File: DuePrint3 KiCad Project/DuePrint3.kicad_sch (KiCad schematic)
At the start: 49 parts, among them J1 MF3.0-2x12-430452412, J10 436500215, J11 M20-9990245, J12 M20-9990245, J13 EHT-125-01-S-D, J14 EHT-110-01-S-D, J15 EHT-125-01-S-D, J2 PPPC161LFBN-RC, J3 PPPC161LFBN-RC, J4 6P2C, J5 6P2C, J6 M20-9990345, J7 436500215, J8 436500815, J9 MF3.0-2x9-430451812, U1 SN74AHCT125DR

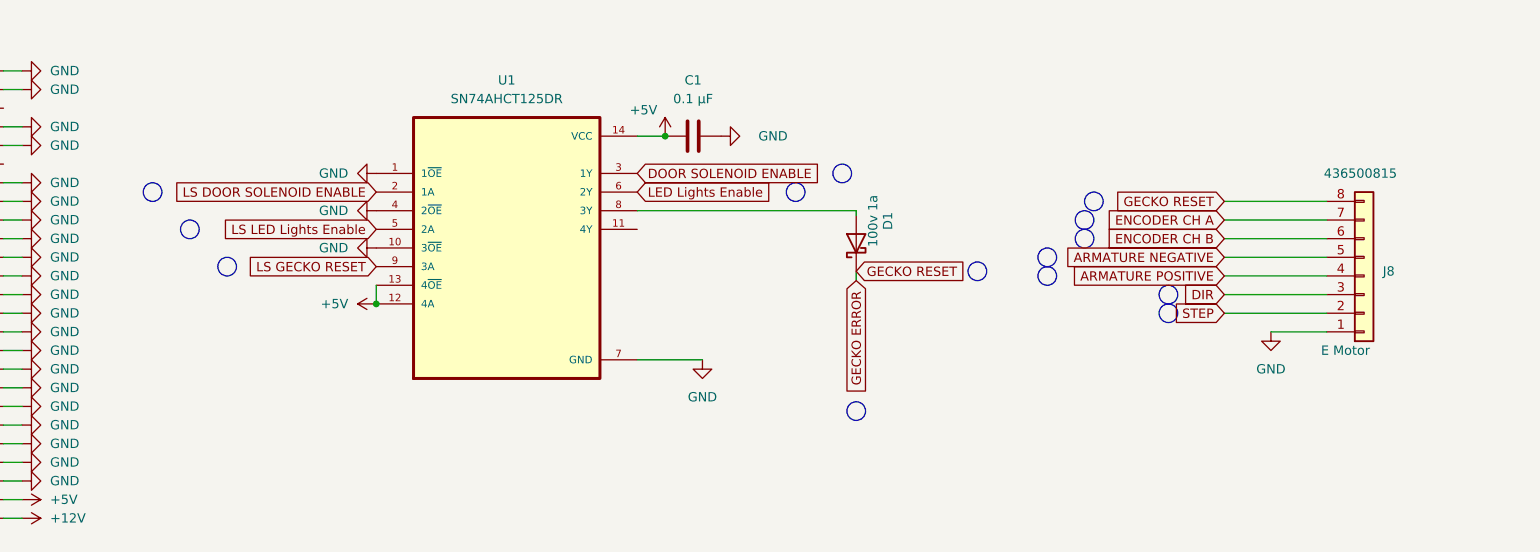
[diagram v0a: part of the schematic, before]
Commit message: Level shifter
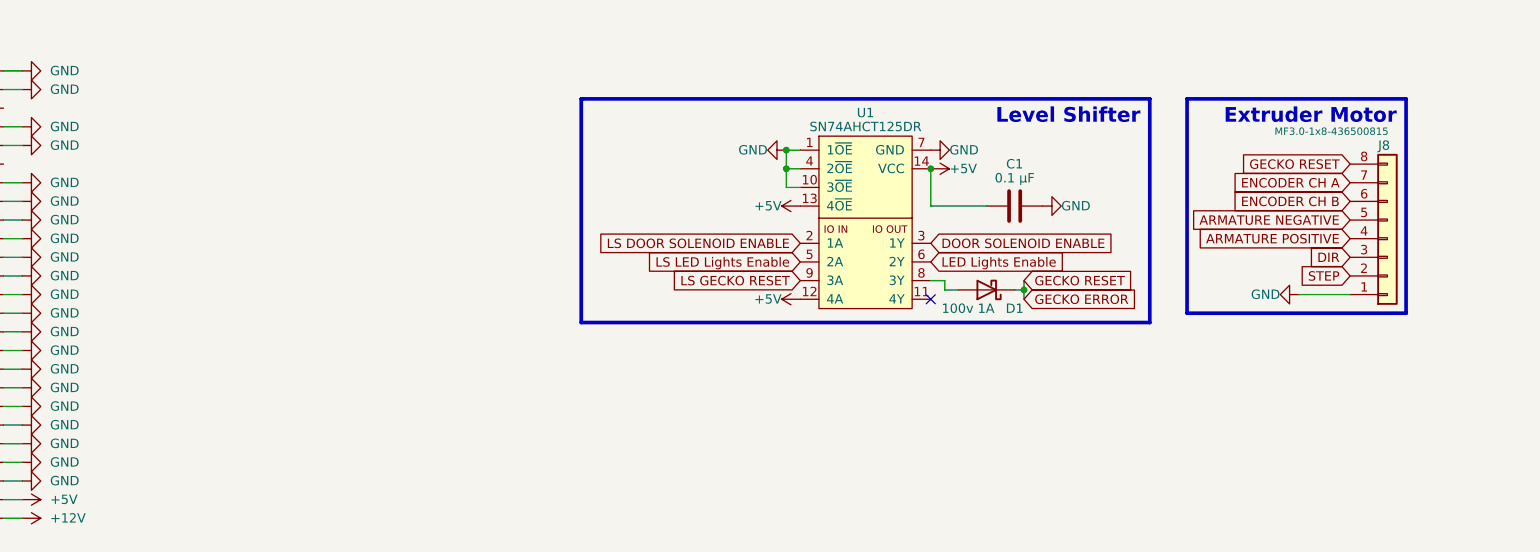
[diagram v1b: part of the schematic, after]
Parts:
- D1: value 100v 1a -> 100v 1A
- J8: value 436500815 -> MF3.0-1x8-436500815; Device E Motor -> (none)
- U1: footprint Stratasys Adapter:SOIC127P600X175-14N -> PCM_Package_SO_AKL:SOIC-14_3.9x8.7mm_P1.27mm
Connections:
- no-connect marks 10 -> 11
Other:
- note added: "Extruder Motor"
- note added: "Level Shifter"
- moved on the sheet: C1, D1, J8

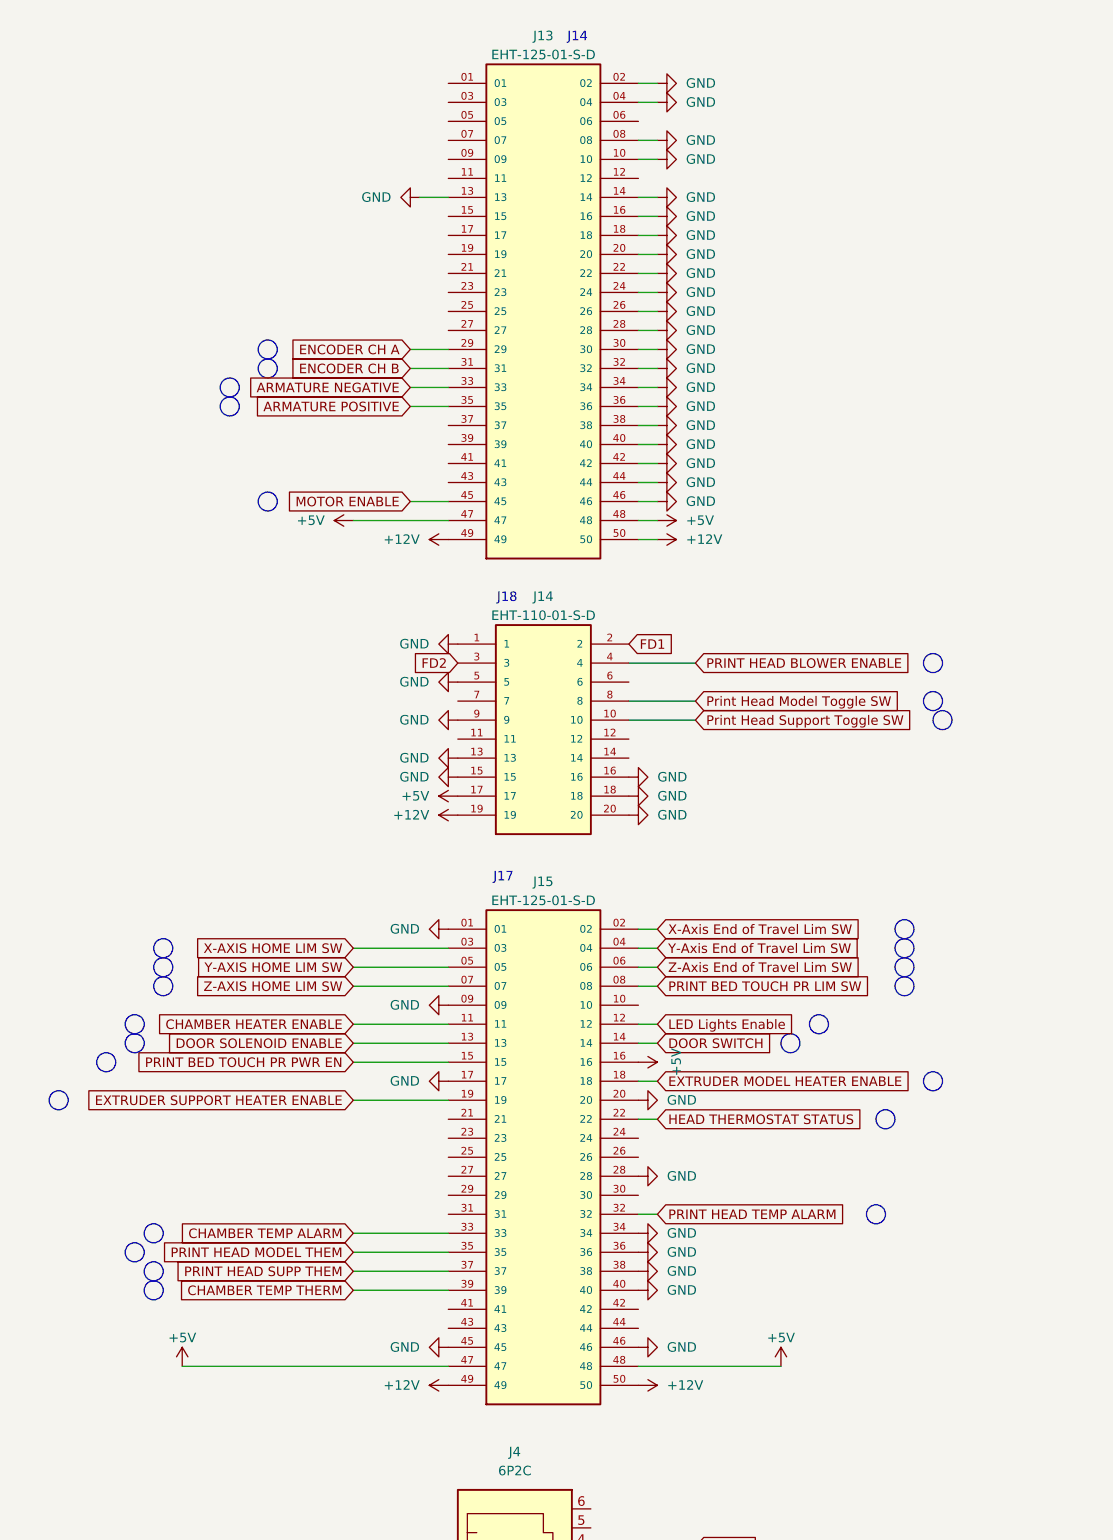
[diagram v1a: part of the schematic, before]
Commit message: PDB Connectors
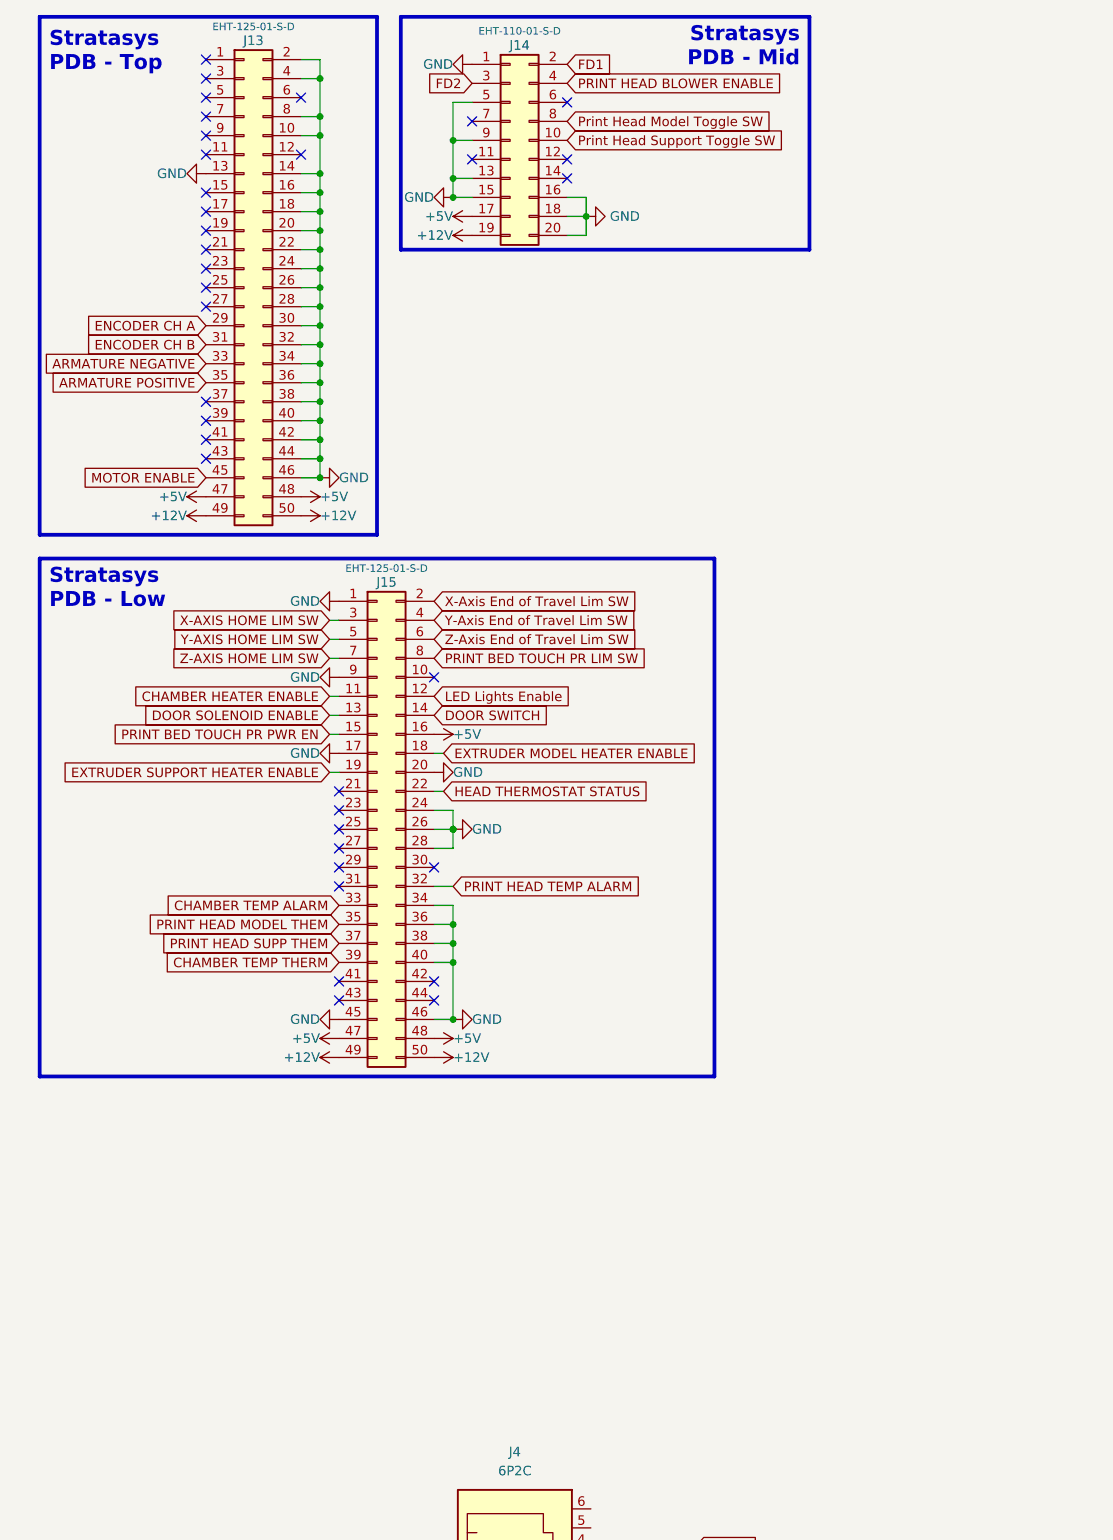
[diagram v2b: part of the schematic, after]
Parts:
- removed J13, J15: EHT-125-01-S-D, EHT-125-01-S-D:SAMTEC_EHT-125-01-S-D, symbol EHT-125-01-S-D:EHT-125-01-S-D
- removed J14: EHT-110-01-S-D, EHT-110-01-XX-D:EHT-110-01-XX-D, symbol EHT-110-01-XX-D:EHT-110-01-XX-D
- added J13, J15: EHT-125-01-S-D, EHT-125-01-S-D:SAMTEC_EHT-125-01-S-D, symbol Connector_Generic:Conn_02x25_Odd_Even
- added J14: EHT-110-01-S-D, EHT-110-01-XX-D:EHT-110-01-XX-D, symbol Connector_Generic:Conn_02x10_Odd_Even
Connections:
- net +12V: now also J13.49 (Pin_49), J13.50 (Pin_50), J14.19 (Pin_19), J15.49 (Pin_49), J15.50 (Pin_50)
- net +5V: now also J13.47 (Pin_47), J13.48 (Pin_48), J14.17 (Pin_17), J15.16 (Pin_16), J15.47 (Pin_47), J15.48 (Pin_48)
- net ARMATURE NEGATIVE: now also J13.33 (Pin_33)
- net ARMATURE POSITIVE: now also J13.35 (Pin_35)
- net CHAMBER HEATER ENABLE: now also J15.11 (Pin_11)
- net CHAMBER TEMP ALARM: now also J15.33 (Pin_33)
- net CHAMBER TEMP THERM: now also J15.39 (Pin_39)
- net DOOR SOLENOID ENABLE: now also J15.13 (Pin_13)
- net DOOR SWITCH: now also J15.14 (Pin_14)
- net EMHE PWM: now also J15.18 (Pin_18)
- net ENCODER CH A: now also J13.29 (Pin_29)
- net ENCODER CH B: now also J13.31 (Pin_31)
- net ESHE PWM: now also J15.19 (Pin_19)
- net FD1: now also J14.2 (Pin_2)
- net FD2: now also J14.3 (Pin_3)
- net GND: now also J13.10 (Pin_10), J13.13 (Pin_13), J13.14 (Pin_14), J13.16 (Pin_16), J13.18 (Pin_18), J13.2 (Pin_2), J13.20 (Pin_20), J13.22 (Pin_22), J13.24 (Pin_24), J13.26 (Pin_26), J13.28 (Pin_28), J13.30 (Pin_30), J13.32 (Pin_32), J13.34 (Pin_34), J13.36 (Pin_36), J13.38 (Pin_38), J13.4 (Pin_4), J13.40 (Pin_40), J13.42 (Pin_42), J13.44 (Pin_44), J13.46 (Pin_46), J13.8 (Pin_8), J14.1 (Pin_1), J14.13 (Pin_13), J14.15 (Pin_15), J14.16 (Pin_16), J14.18 (Pin_18), J14.20 (Pin_20), J14.5 (Pin_5), J14.9 (Pin_9), J15.1 (Pin_1), J15.17 (Pin_17), J15.20 (Pin_20), J15.24 (Pin_24), J15.26 (Pin_26), J15.28 (Pin_28), J15.34 (Pin_34), J15.36 (Pin_36), J15.38 (Pin_38), J15.40 (Pin_40), J15.45 (Pin_45), J15.46 (Pin_46), J15.9 (Pin_9)
- net HEAD THERMOSTAT STATUS: now also J15.22 (Pin_22)
- net LED Lights Enable: now also J15.12 (Pin_12)
- net MOTOR ENABLE: now also J13.45 (Pin_45)
- net PBTPE PWM: now also J15.15 (Pin_15)
- net PHBE PWM: now also J14.4 (Pin_4)
- net PRINT BED TOUCH PR LIM SW: now also J15.8 (Pin_8)
- net PRINT HEAD MODEL THEM: now also J15.35 (Pin_35)
- net PRINT HEAD SUPP THEM: now also J15.37 (Pin_37)
- net PRINT HEAD TEMP ALARM: now also J15.32 (Pin_32)
- net Print Head Model Toggle SW: now also J14.8 (Pin_8)
- net Print Head Support Toggle SW: now also J14.10 (Pin_10)
- net X-AXIS HOME LIM SW: now also J15.3 (Pin_3)
- net X-Axis End of Travel Lim SW: now also J15.2 (Pin_2)
- net Y-AXIS HOME LIM SW: now also J15.5 (Pin_5)
- net Y-Axis End of Travel Lim SW: now also J15.4 (Pin_4)
- net Z-AXIS HOME LIM SW: now also J15.7 (Pin_7)
- net Z-Axis End of Travel Lim SW: now also J15.6 (Pin_6)
- no-connect marks 11 -> 47
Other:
- note added: "Stratasys PDB - Low"
- note added: "Stratasys PDB - Mid"
- note added: "Stratasys PDB - Top"
- note removed: "J14"
- note removed: "J17"
- note removed: "J18"

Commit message: The Rest Of The Schematic
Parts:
- removed J10, J7: 436500215, Connector_Molex:Molex_Micro-Fit_3.0_43650-0215_1x02_P3.00mm_Vertical, symbol Connector:Conn_01x02_Pin
- removed J11, J12: M20-9990245, Connector_PinHeader_2.54mm:PinHeader_1x02_P2.54mm_Vertical, symbol Connector:Conn_01x02_Pin
- removed J2, J3: PPPC161LFBN-RC, Connector_PinSocket_2.54mm:PinSocket_1x16_P2.54mm_Vertical, symbol Connector:Conn_01x16_Socket
- removed J6: M20-9990345, Connector_PinHeader_2.54mm:PinHeader_1x03_P2.54mm_Vertical, symbol Connector:Conn_01x03_Pin
- added J10, J7: MF3.0-1x2-436500215, Connector_Molex:Molex_Micro-Fit_3.0_43650-0215_1x02_P3.00mm_Vertical, symbol Connector_Generic:Conn_01x02
- added J11, J12: 2.54Header-1x2-M, Connector_PinHeader_2.54mm:PinHeader_1x02_P2.54mm_Vertical, symbol Connector_Generic:Conn_01x02
- added J2, J3: 2.54Header-1x16-F, symbol Connector_Generic:Conn_01x16
- added J6: 2.54Header-1x3-M, symbol Connector_Generic:Conn_01x03
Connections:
- net +12V: now also J10.2 (Pin_2)
- net +5V: now also R24.2, J2.15 (Pin_15), J3.16 (Pin_16), J7.2 (Pin_2); no longer R24.1
- net CAN0H: now also J3.1 (Pin_1), J6.3 (Pin_3)
- net CAN0L: now also J3.2 (Pin_2), J6.1 (Pin_1)
- net DIR: now also J2.11 (Pin_11)
- net DOOR SWITCH: now also J2.7 (Pin_7)
- net FD1: now also J11.1 (Pin_1)
- net FD2: now also J12.1 (Pin_1)
- net GECKO ERROR: now also J2.5 (Pin_5)
- net GND: now also J10.1 (Pin_1), J2.16 (Pin_16), J7.1 (Pin_1)
- net HEAD THERMOSTAT STATUS: now also J2.6 (Pin_6)
- net Print Head Model Toggle SW: now also J3.8 (Pin_8)
- net Print Head Support Toggle SW: now also J2.8 (Pin_8)
- net STEP: now also J2.12 (Pin_12)
- net at R17.2: now also J6.2 (Pin_2)
- net at R25.2: now also J12.2 (Pin_2), J2.3 (Pin_3)
- new net: J11.2 (Pin_2), J2.13 (Pin_13), R24.1
- no-connect marks 47 -> 75
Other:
- note added: "4mm Holes"
- note added: "CAN-FD RJ11 Ports"
- note added: "Power Access"
- note added: "STM32 Extruder"
- note added: "Sammy C21 MCU Module"
- note removed: "Extruder Motor"
- moved on the sheet: C1, D1, H1, H2, H3, H4, H5, H6, J1, J14, J15, J4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
